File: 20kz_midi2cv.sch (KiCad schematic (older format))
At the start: 17 parts

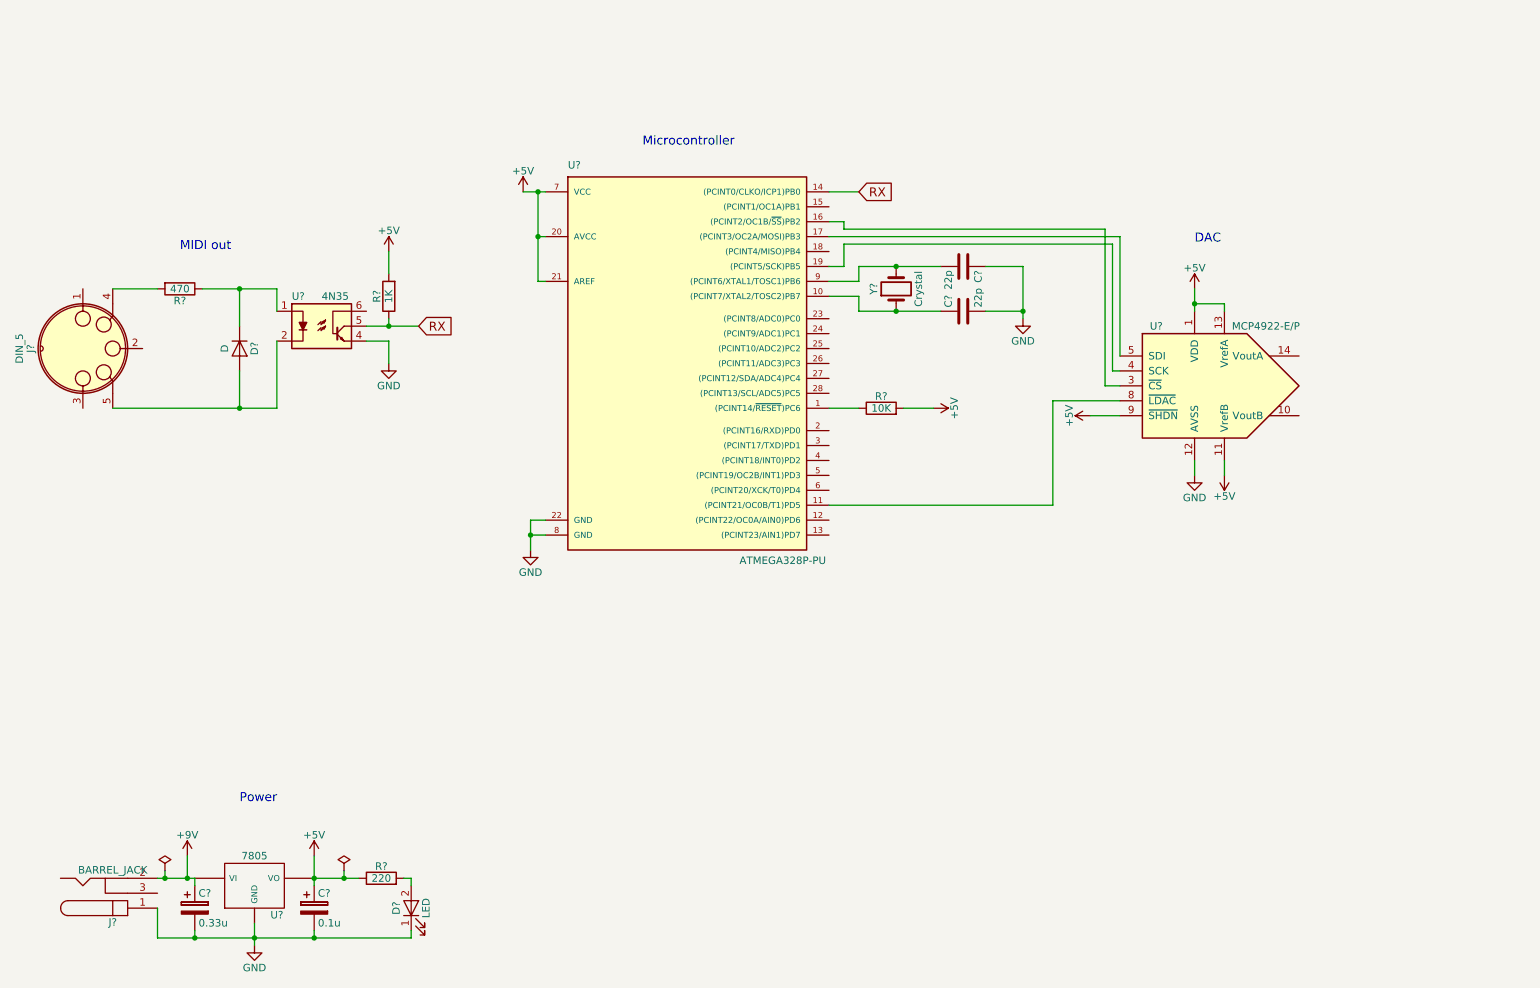
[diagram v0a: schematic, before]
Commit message: ...
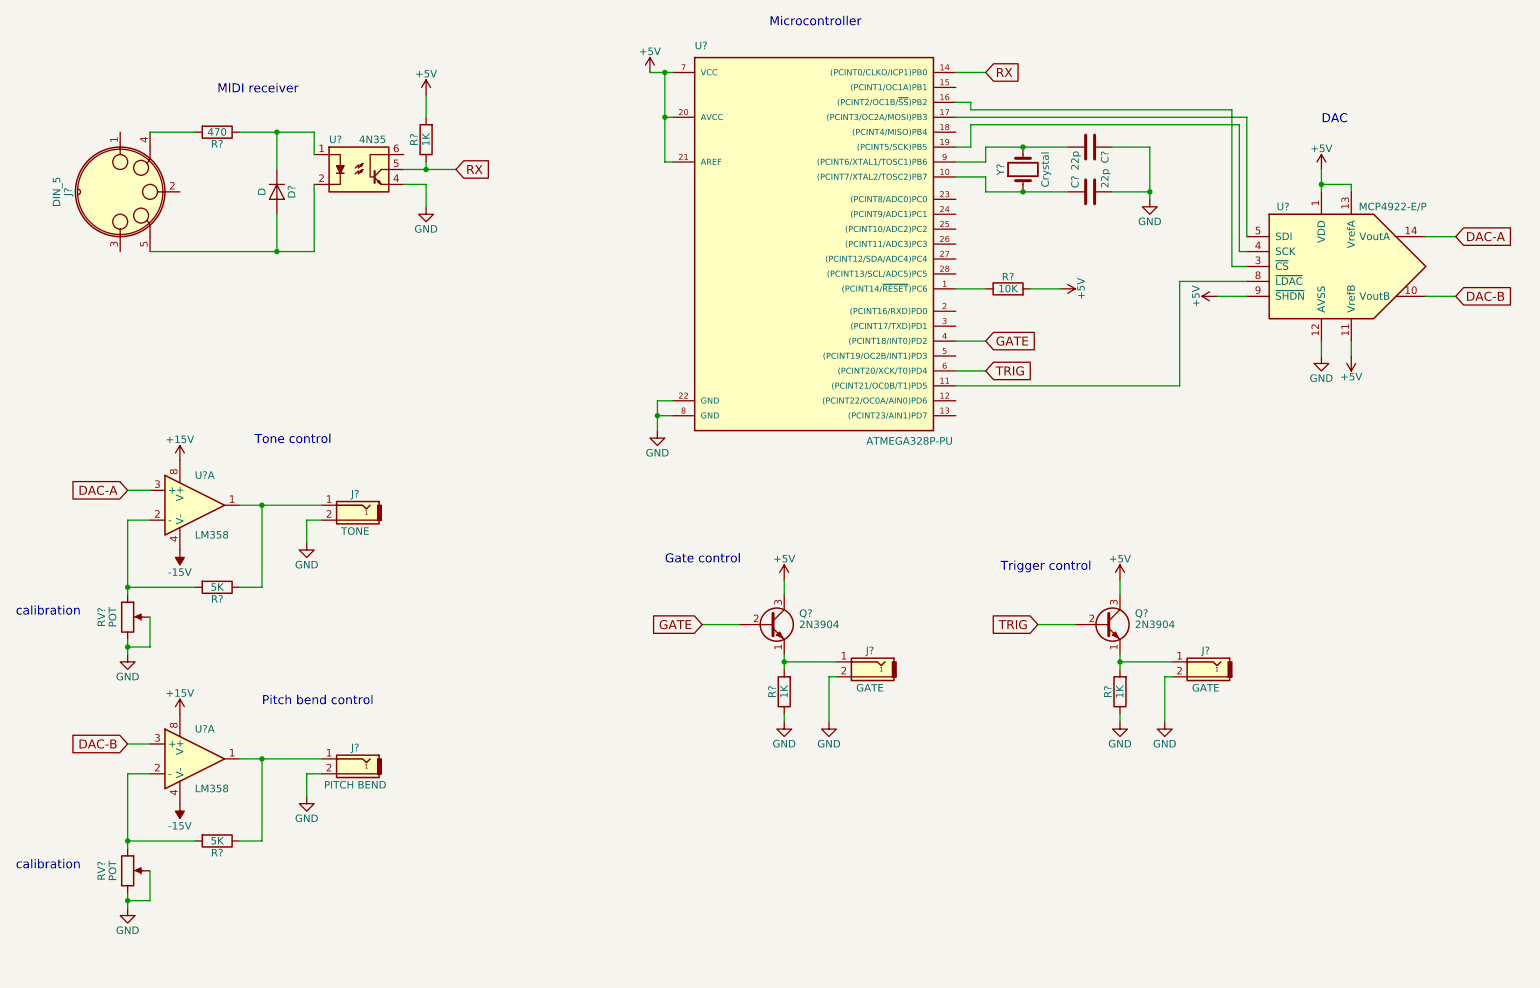
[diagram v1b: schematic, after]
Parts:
- removed C?: 0.33u, symbol CP
- removed C?: 0.1u, symbol CP
- removed D?: LED, symbol LED
- removed J?: BARREL_JACK, symbol BARREL_JACK
- removed R?: 220, symbol R
- removed U?: 7805, symbol 7805
- added J?: TONE, symbol Audio-Jack-2
- added J?: PITCH BEND, symbol Audio-Jack-2
- added J? (x2): GATE, symbol Audio-Jack-2
- added Q? (x2): 2N3904, TO_SOT_Packages_THT:TO-92_Molded_Narrow, symbol 2N3904
- added R? (x2): 5K, symbol R
- added R? (x2): 1K, symbol R
- added RV? (x2): POT, symbol POT
- added U? (x2): LM358, symbol LM358
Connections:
- net +5V: now also Q?.3 (C), Q?.3 (C)
- net GND: now also J?.2, J?.2, J?.2, J?.2, R?.1, R?.1, RV?.2, RV?.2, RV?.3, RV?.3
- net GATE: now reaches U?.4 ((PCINT18/INT0)PD2)
- net GATE: now also Q?.2 (B)
- net TRIG: now reaches U?.6 ((PCINT20/XCK/T0)PD4)
- net TRIG: now also Q?.2 (B)
- net DAC-B: now reaches U?.10 (VoutB)
- net DAC-B: now also U?.3 (+)
- net DAC-A: now reaches U?.14 (VoutA)
- net DAC-A: now also U?.3 (+)
- new net: J?.1, R?.1, U?.1 (x2)
- new net: R?.2, RV?.1, U?.2 (-) (x2)
- new net: J?.1, Q?.1 (E), R?.2 (x2)
- new net +15V: U?.8 (V+), U?.8 (V+)
- new net -15V: U?.4 (V-), U?.4 (V-)
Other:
- note added: "Gate control"
- note added: "MIDI receiver"
- note added: "Pitch bend control"
- note added: "Tone control"
- note added: "Trigger control"
- note added: "calibration"
- note removed: "MIDI out"
- note removed: "Power\n"
- moved on the sheet: C?, D?, J?, R?, U?, Y?
